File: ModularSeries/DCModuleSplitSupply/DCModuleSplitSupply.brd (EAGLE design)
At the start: 82 x 36 mm, 26 parts, among them J1 2XMOLEX, J2 4XMOLEX, J3 4XMOLEX, J4 4XMOLEX, J5 4XMOLEX, J6 2XMOLEX, J7 2XMOLEX, J8 4XMOLEX

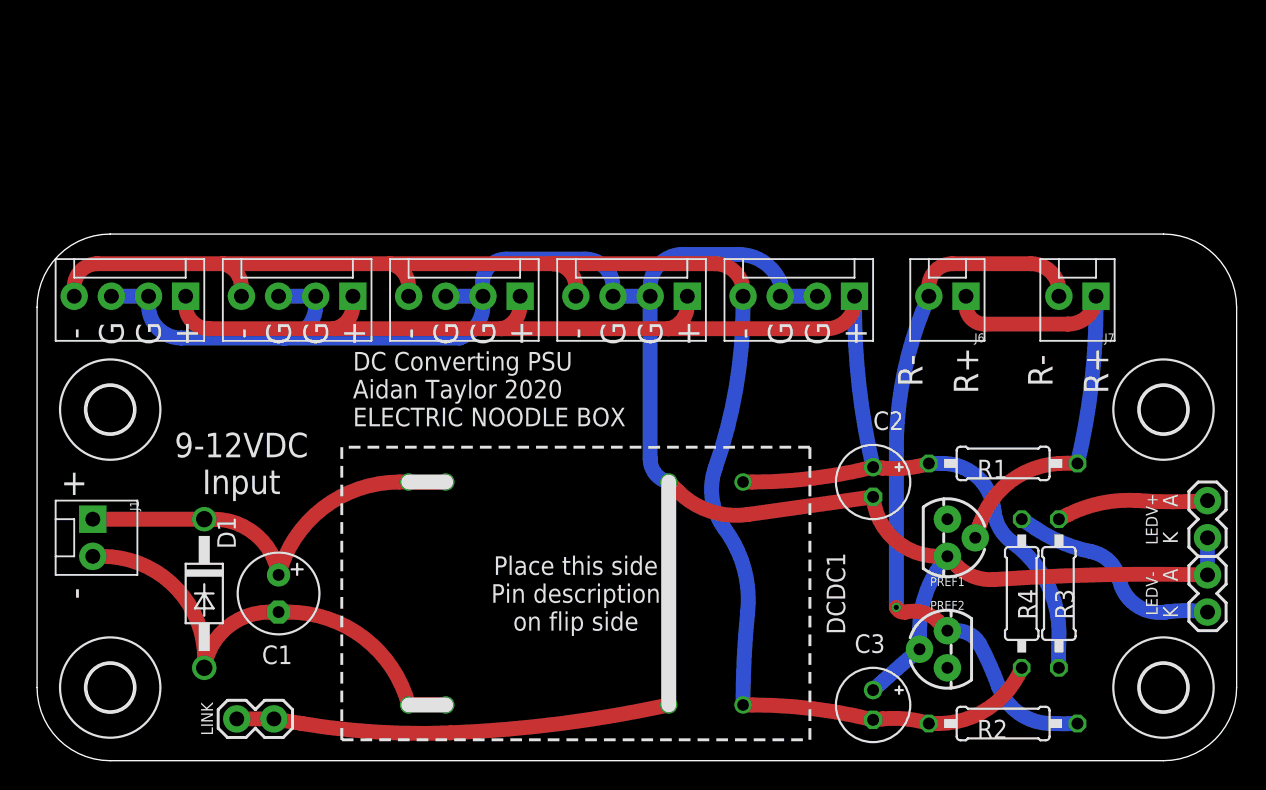
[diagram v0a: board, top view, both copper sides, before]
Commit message: DC Split Supply layout revision
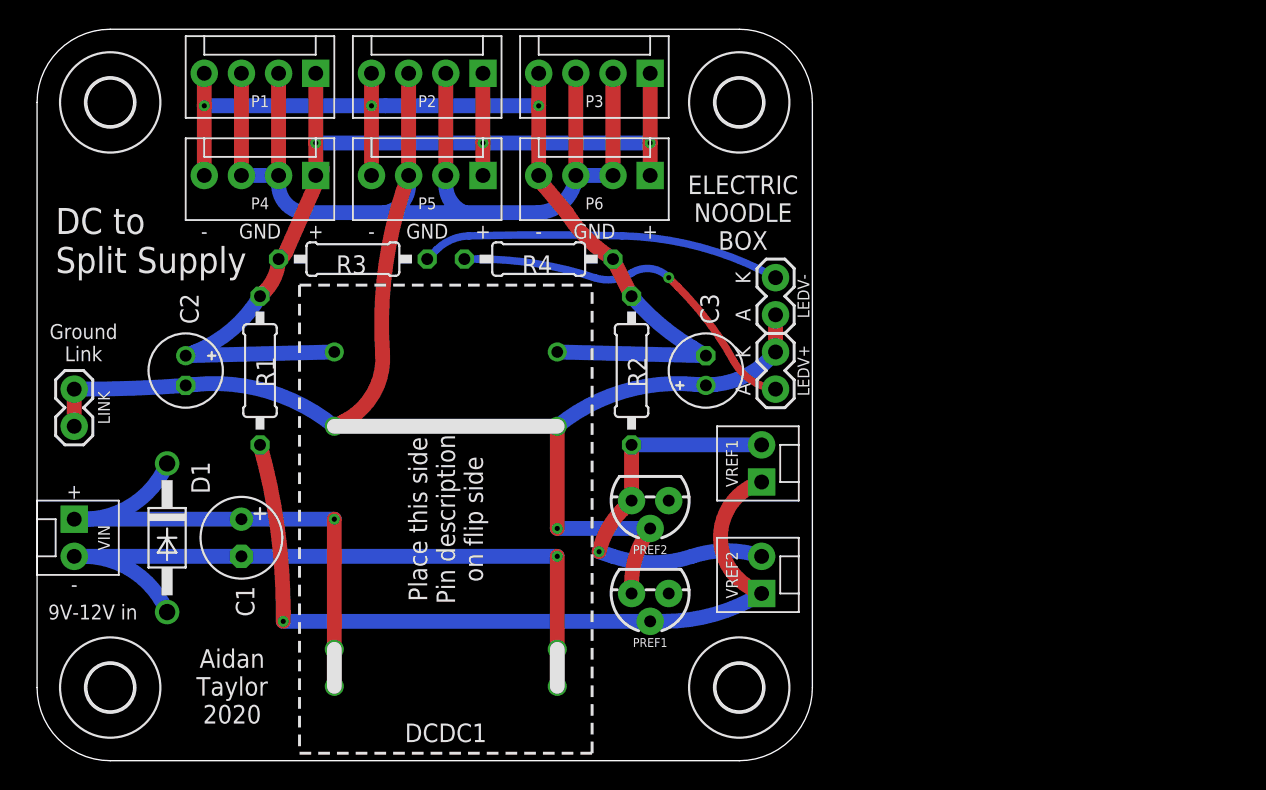
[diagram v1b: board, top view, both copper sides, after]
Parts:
- removed J1, J6, J7: 2XMOLEX, ElectricNoodleBox:MOLEX-1X2
- removed J2, J3, J4, J5, J8: 4XMOLEX, ElectricNoodleBox:MOLEX-1X4
- added P1, P2, P3, P4, P5, P6: 4XMOLEX, ElectricNoodleBox:MOLEX-1X4
- added VIN, VREF1, VREF2: 2XMOLEX, ElectricNoodleBox:MOLEX-1X2
- moved H4 75.0 mm to (5.00, 45.0)
- moved R3 53.4 mm to (21.6, 34.3), turned to 180 degrees
- moved R1 51.2 mm to (15.2, 26.7), turned to 270 degrees
- moved H3 49.4 mm to (48.0, 45.0)
- moved C2 47.6 mm to (10.2, 26.7)
- moved H2 43.0 mm to (48.0, 5.00)
- moved R4 40.2 mm to (34.3, 34.3), turned to 0 degrees
- moved R2 35.0 mm to (40.6, 26.7), turned to 270 degrees
- moved LEDV+ 33.2 mm to (50.5, 30.5)
- moved LEDV- 33.2 mm to (50.5, 27.9)
- moved C3 25.6 mm to (45.7, 26.7), turned to 90 degrees
- moved LINK 22.9 mm to (2.54, 22.9), turned to 90 degrees
- moved PREF2 22.7 mm to (41.9, 17.8), turned to 180 degrees
- moved PREF1 20.7 mm to (41.9, 11.4), turned to 180 degrees
- moved H1 19.0 mm to (5.00, 5.00)
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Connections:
- net +10VREF: now also VREF1.1, VREF2.1; no longer J6.1, J7.1
- net +12V: now also P1.1, P2.1, P3.1, P4.1, P5.1, P6.1; no longer J2.1, J3.1, J4.1, J5.1, J8.1
- net -10VREF: now also VREF1.2, VREF2.2; no longer J6.2, J7.2
- net -12V: now also P1.4, P2.4, P3.4, P4.4, P5.4, P6.4; no longer J2.4, J3.4, J4.4, J5.4, J8.4
- net AGND: now also P1.2, P1.3, P2.2, P2.3, P3.2, P3.3, P4.2, P4.3, P5.2, P5.3, P6.2, P6.3; no longer J2.2, J2.3, J3.2, J3.3, J4.2, J4.3, J5.2, J5.3, J8.2, J8.3
- net N$4: now also VIN.1; no longer J1.1
- net N$5: now also VIN.2; no longer J1.2
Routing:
- net -12V: track 104.9 -> 71.0 mm, vias 0 -> 3
- net +12V: track 98.1 -> 70.9 mm, vias 0 -> 3
- net +10VREF: track 31.4 -> 53.2 mm, vias 0 -> 1
- net -10VREF: track 48.5 -> 28.0 mm
- net N$5: track 31.1 -> 48.8 mm, vias 0 -> 1
- net N$2: track 10.3 -> 24.7 mm
- net AGND: track 177.5 -> 166.6 mm, vias 0 -> 1
- net N$3: track 14.7 -> 24.8 mm, vias 0 -> 1
- net N$4: track 27.7 -> 36.1 mm, vias 0 -> 1
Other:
- board size 82 x 36 mm -> 53 x 50 mm
- board text added: "9V-12V in"
- board text added: "Aidan Taylor 2020"
- board text added: "DC to Split Supply"
- board text added: "ELECTRIC NOODLE BOX"
- board text added: "GND"
- board text added: "Ground Link"
- board text removed: "9-12VDC Input"
- board text removed: "DC Converting PSU Aidan Taylor 2020 ELECTRIC NOODLE BOX"
- board text removed: "G"
- board text removed: "R+"
- board text removed: "R-"
